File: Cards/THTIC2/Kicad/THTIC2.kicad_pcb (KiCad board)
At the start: 2 copper layers, 50.3 x 24.1 mm, 25 parts, among them J1 Conn_01x04_Pin, J2 Plasma 300V, U1 B0509S-1WR3, U2 ISO1540, U3 ADS1014IDGS, U4 AMS1117-5, U5 LMV321

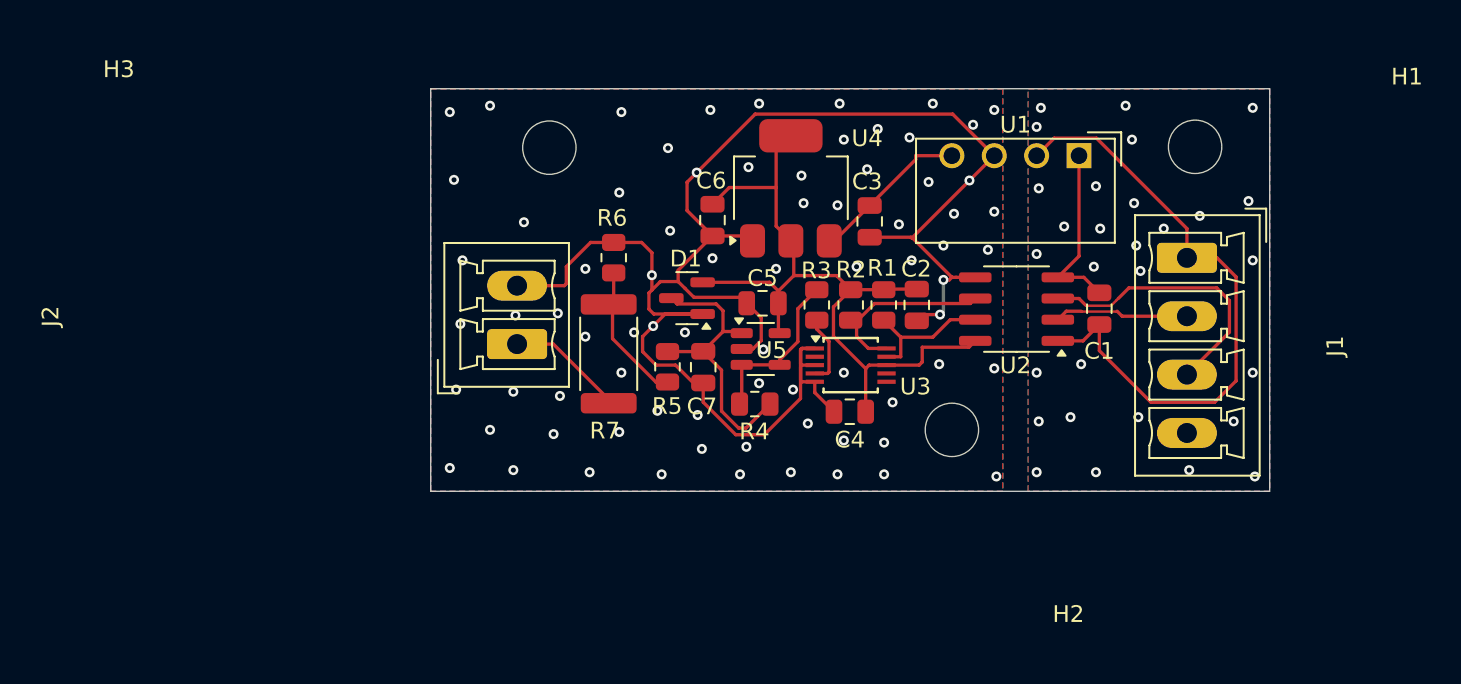
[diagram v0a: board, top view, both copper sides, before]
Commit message: Final version of THTIC2
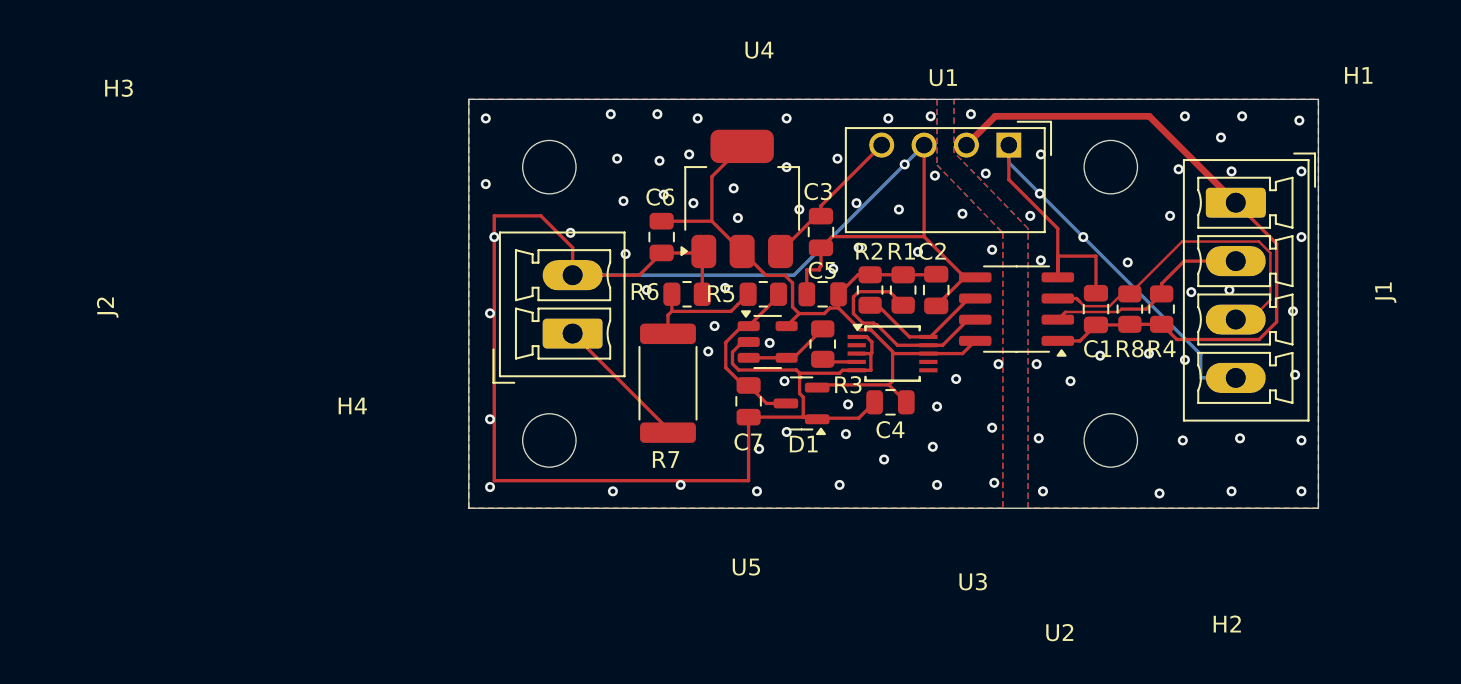
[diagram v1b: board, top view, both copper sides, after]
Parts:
- added H4: MountingHole, MountingHole:MountingHole_3.2mm_M3, F.Cu at (155.2, 104.8)
- added R8: 2k2, Resistor_SMD:R_0805_2012Metric, F.Cu at (190.0, 96.9)
- R4: value nP -> 2k2
- R6: value 1k27 -> 2k1
- moved R4 25.0 mm to (191.9, 96.9), turned to 90 degrees
- moved H2 9.55 mm to (188.8, 104.8)
- moved D1 9.33 mm to (170.3, 102.6)
- moved R5 7.21 mm to (168.0, 96.0), turned to 180 degrees
- moved H1 5.20 mm to (188.8, 88.4)
- moved R6 4.92 mm to (163.4, 96.0), turned to 0 degrees
- moved J1 4.41 mm to (196.3, 90.5)
- moved U1 4.25 mm to (182.7, 87.1)
- moved R7 3.97 mm to (162.3, 101.3)
- moved C5 3.64 mm to (171.6, 96.0)
- moved C7 3.40 mm to (167.1, 102.4)
- moved J2 3.39 mm to (156.6, 98.4)
- moved C6 3.21 mm to (161.9, 92.6)
- moved C3 2.99 mm to (171.5, 92.3)
- moved U4 2.99 mm to (166.8, 90.3)
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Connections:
- C7 pad 1: Net-(D2-COM) -> Net-(D1-COM)
- D1 pad 3: Net-(D2-COM) -> Net-(D1-COM)
- R3 pad 2: Net-(U7--) -> Net-(U5--)
- R4 pad 1: Net-(U7--) -> 5V
- R4 pad 2: Net-(D2-COM) -> Net-(J1-Pin_2)
- R5 pad 1: Net-(D2-COM) -> Net-(D1-COM)
- U5 pad 1: Net-(D2-COM) -> Net-(D1-COM)
- U5 pad 3: Net-(U7--) -> Net-(U5--)
- U5 pad 4: Net-(U7--) -> Net-(U5--)
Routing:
- net GND: track 10.7 -> 35.7 mm, vias 29 -> 34
- net GND_ISO: track 105.5 -> 124.2 mm, vias 76 -> 56
- net Net-(D2-COM): track 17.6 -> 0.00 mm
- net Net-(D1-COM): track 0.00 -> 10.4 mm
- net Net-(U7--): track 10.1 -> 0.00 mm
- net Net-(U5--): track 0.00 -> 5.16 mm
- net Net-(U2-SDA2): track 8.37 -> 13.2 mm
- net Net-(J1-Pin_2): track 8.09 -> 12.5 mm
- net 5V: track 37.6 -> 41.5 mm
- net Net-(J1-Pin_3): track 16.7 -> 20.3 mm
- net Net-(U2-SCL2): track 11.1 -> 8.04 mm
- net Net-(U3-AIN0): track 4.30 -> 2.10 mm
- net VCC_ISO: track 46.1 -> 44.9 mm
- net Net-(J2-Pin_1): track 7.19 -> 8.31 mm
- net Net-(U1-+Vout): track 9.98 -> 9.07 mm
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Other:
- board size 50.3 x 24.1 mm -> 50.9 x 24.5 mm
- board text added: "MetalMusings THTIC2 Feb 2025"
- board text removed: "MetalMusings THTIC2 prototype 1 Feb 2025"
